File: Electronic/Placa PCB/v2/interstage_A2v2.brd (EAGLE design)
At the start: 82.5 x 29 mm, 11 parts, among them J1 0532611271, J3 0532611271, Q1 PMV16XNR, U1 LM70CIMM-3, U2 LM70CIMM-3

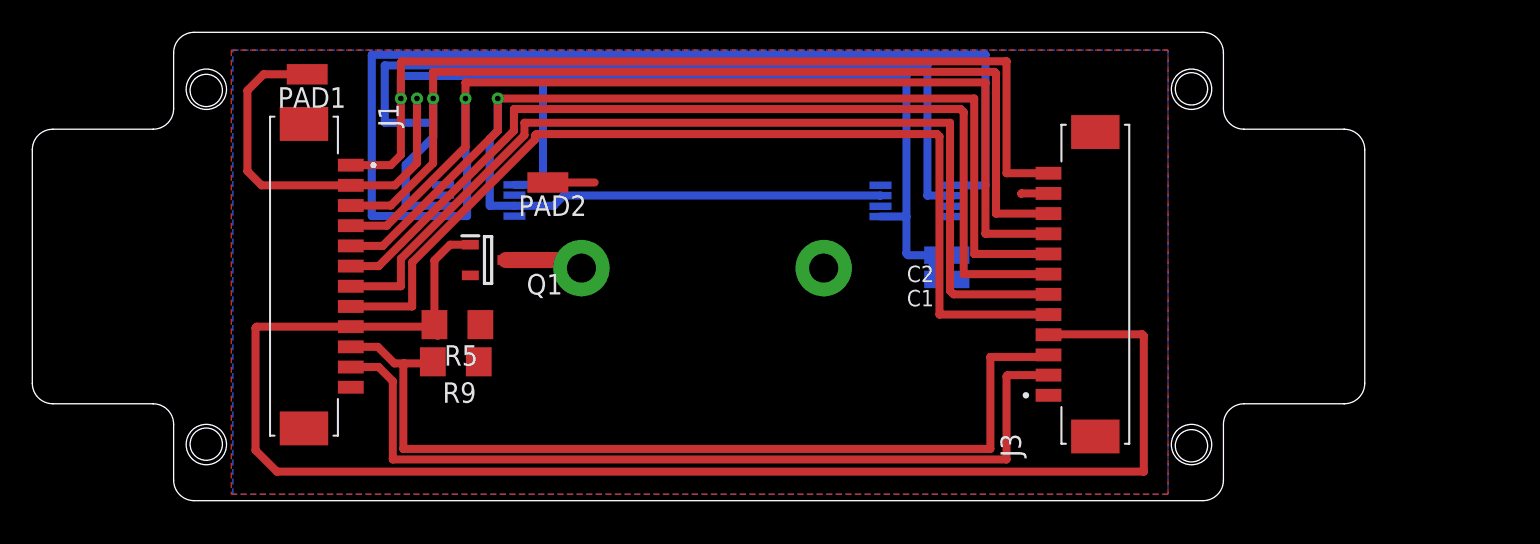
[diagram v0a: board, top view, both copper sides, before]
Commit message: Avance
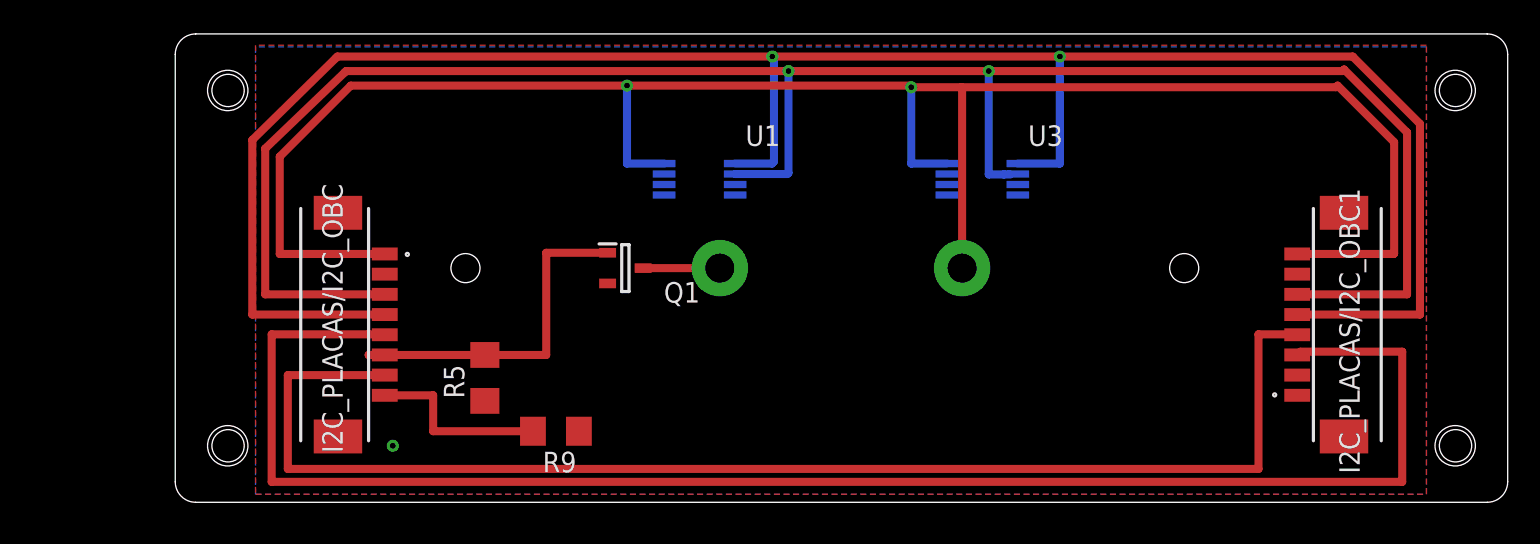
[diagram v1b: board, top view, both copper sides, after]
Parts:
- removed C1, C2: 0.1pF, rcl:C0603K
- removed J1, J3: 0532611271, picoblade:MOLEX_0532611271
- removed PAD1, PAD2: WIREPADSMD1,27-254, wirepad:SMD1,27-2,54
- removed U2: LM70CIMM-3, LM70CIMM-3:SOP65P490X110-8N
- added I2C_PLACAS/I2C_OBC, I2C_PLACAS/I2C_OBC1: 53261-0871, SamacSys_Parts:53261-0871
- added U3: MCP9808T-E/MS, sensorSPEL:SOP65P490X110-8N
- U1: value LM70CIMM-3 -> MCP9808T-E/MS; device LM70CIMM-3:SOP65P490X110-8N -> sensorSPEL:SOP65P490X110-8N
- moved U1 13.5 mm to (32.5, 20.0)
- moved Q1 8.51 mm to (27.9, 14.5)
- moved R9 7.55 mm to (23.6, 4.40)
- moved R5 3.71 mm to (19.2, 7.70), turned to 90 degrees
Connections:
- removed net AIN1: J1.7, J3.6
- removed net MISO: J1.4, J3.9, U1.1, U2.1
- removed net MOSI: J1.5, J3.8, U1.7, U2.7
- removed net N$3: J3.1
- removed net SCK: J1.3, J3.10, U1.2, U2.2
- removed net T1: J1.9, J3.4, Q1.1, R5.2
- new net SCL: I2C_PLACAS/I2C_OBC.3, I2C_PLACAS/I2C_OBC1.6, U1.2, U3.2
- new net SDA: I2C_PLACAS/I2C_OBC.4, I2C_PLACAS/I2C_OBC1.5, U1.1, U3.1
- net AIN0: now also I2C_PLACAS/I2C_OBC.6, Q1.1, R5.2; no longer J1.8, J3.5
- net GND: now also I2C_PLACAS/I2C_OBC.2, I2C_PLACAS/I2C_OBC1.7, U3.4; no longer C1.2, C2.2, J1.2, J3.11, PAD1.1, PAD2.1, U2.4
- net INT0: now also I2C_PLACAS/I2C_OBC.7, I2C_PLACAS/I2C_OBC1.4; no longer J1.10, J3.3, R9.2
- net OC1A: now also I2C_PLACAS/I2C_OBC.5, I2C_PLACAS/I2C_OBC1.3; no longer J1.6, J3.7
- net T0: now also I2C_PLACAS/I2C_OBC.8, R9.2; no longer J1.11, J3.2
- net VCC: now also I2C_PLACAS/I2C_OBC.1, I2C_PLACAS/I2C_OBC1.8, U1.8, U3.8; no longer C1.1, C2.1, J1.1, J3.12, U1.5, U2.5
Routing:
- net SDA: track 0.00 -> 132.8 mm, vias 0 -> 2
- net MISO: track 129.8 -> 0.00 mm, vias 1 -> 0
- net SCL: track 0.00 -> 124.9 mm, vias 0 -> 2
- net SCK: track 118.1 -> 0.00 mm, vias 1 -> 0
- net T1: track 95.7 -> 0.00 mm
- net MOSI: track 89.1 -> 0.00 mm, vias 1 -> 0
- net AIN1: track 59.3 -> 0.00 mm
- net T0: track 53.8 -> 11.4 mm
- net OC1A: track 58.5 -> 100.8 mm
- net AIN0: track 60.8 -> 22.1 mm
- net GND: track 29.2 -> 0.00 mm
- net INT0: track 55.9 -> 82.7 mm
- net VCC: track 113.2 -> 123.1 mm, vias 1 -> 3
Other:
- outline, holes or cut-outs redrawn
